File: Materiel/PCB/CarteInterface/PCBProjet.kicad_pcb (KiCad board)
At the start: 2 copper layers, 65 x 56 mm, 21 parts

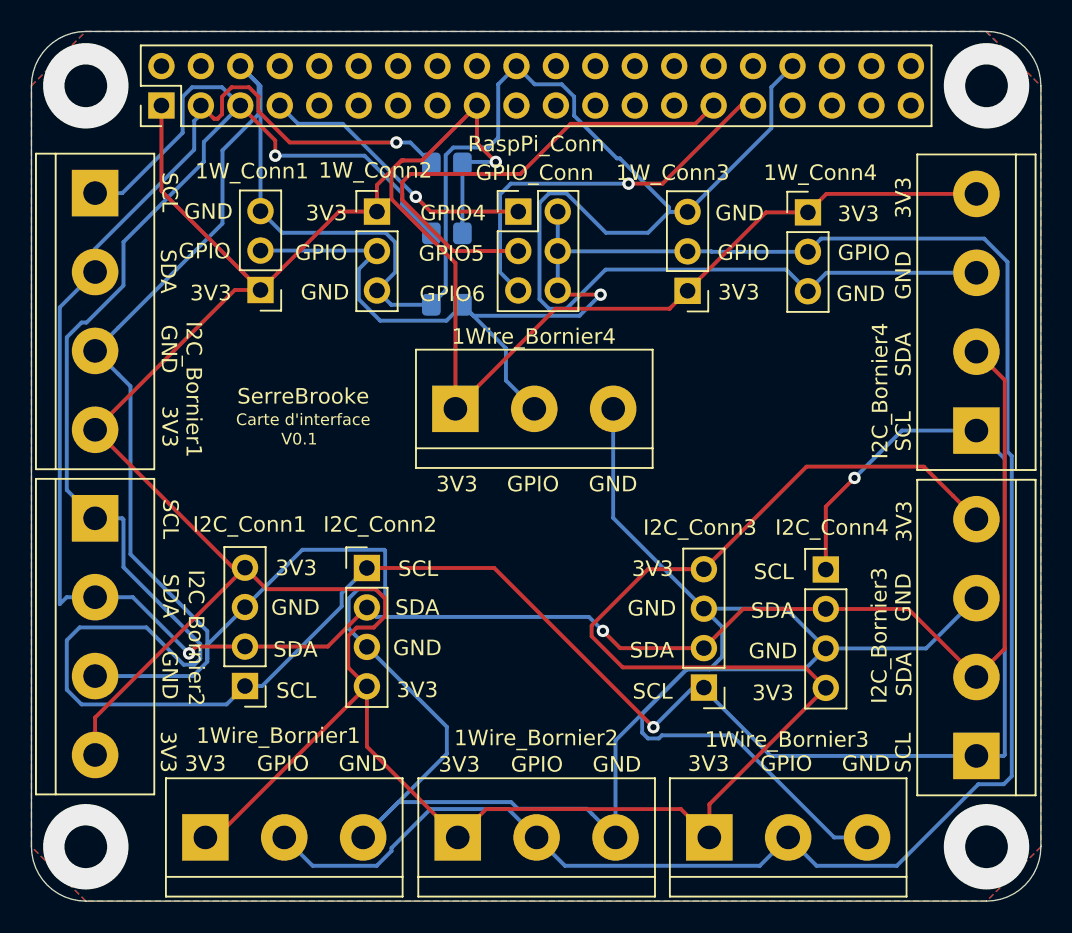
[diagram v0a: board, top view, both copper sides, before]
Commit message: Travailler sur manuel technique
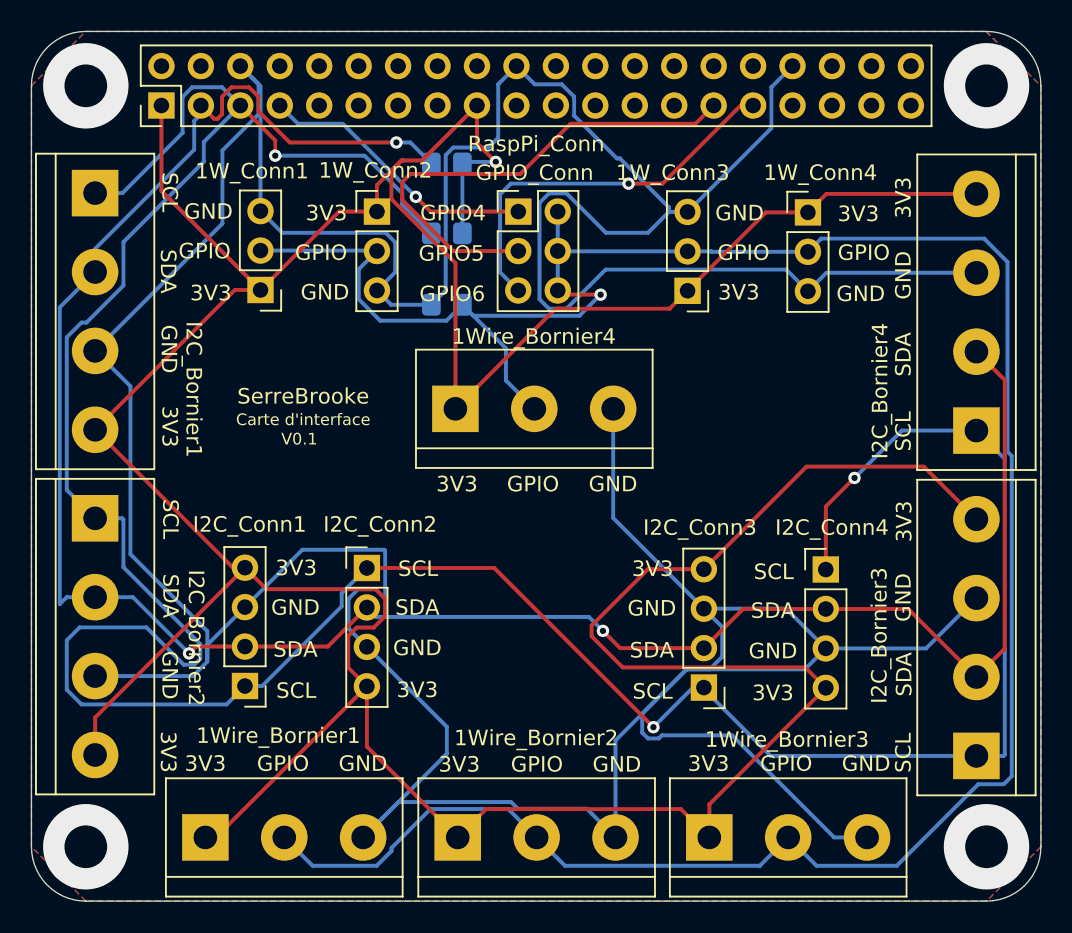
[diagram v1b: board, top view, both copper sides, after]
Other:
- net class Default removed
